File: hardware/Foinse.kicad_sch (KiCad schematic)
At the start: 81 parts, among them J1 ESQ-110-X-X-D, J15 39-29-1048, J3 PJ-063AH, J4 5023860570, J7 FAULT2, J8 FAULT1, Q1 IPD90P04P4L04ATMA1, Q2 IPD90P04P4L04ATMA1, U1 STM32F072C8Tx, U17 LTC4412xS6, U19 TPS56A37RPAR, U4 TJA1051T-3, U5 TPS563203, U6 ACS71240KEXBLT-010B3, U7 ACS71240KEXBLT-010B3

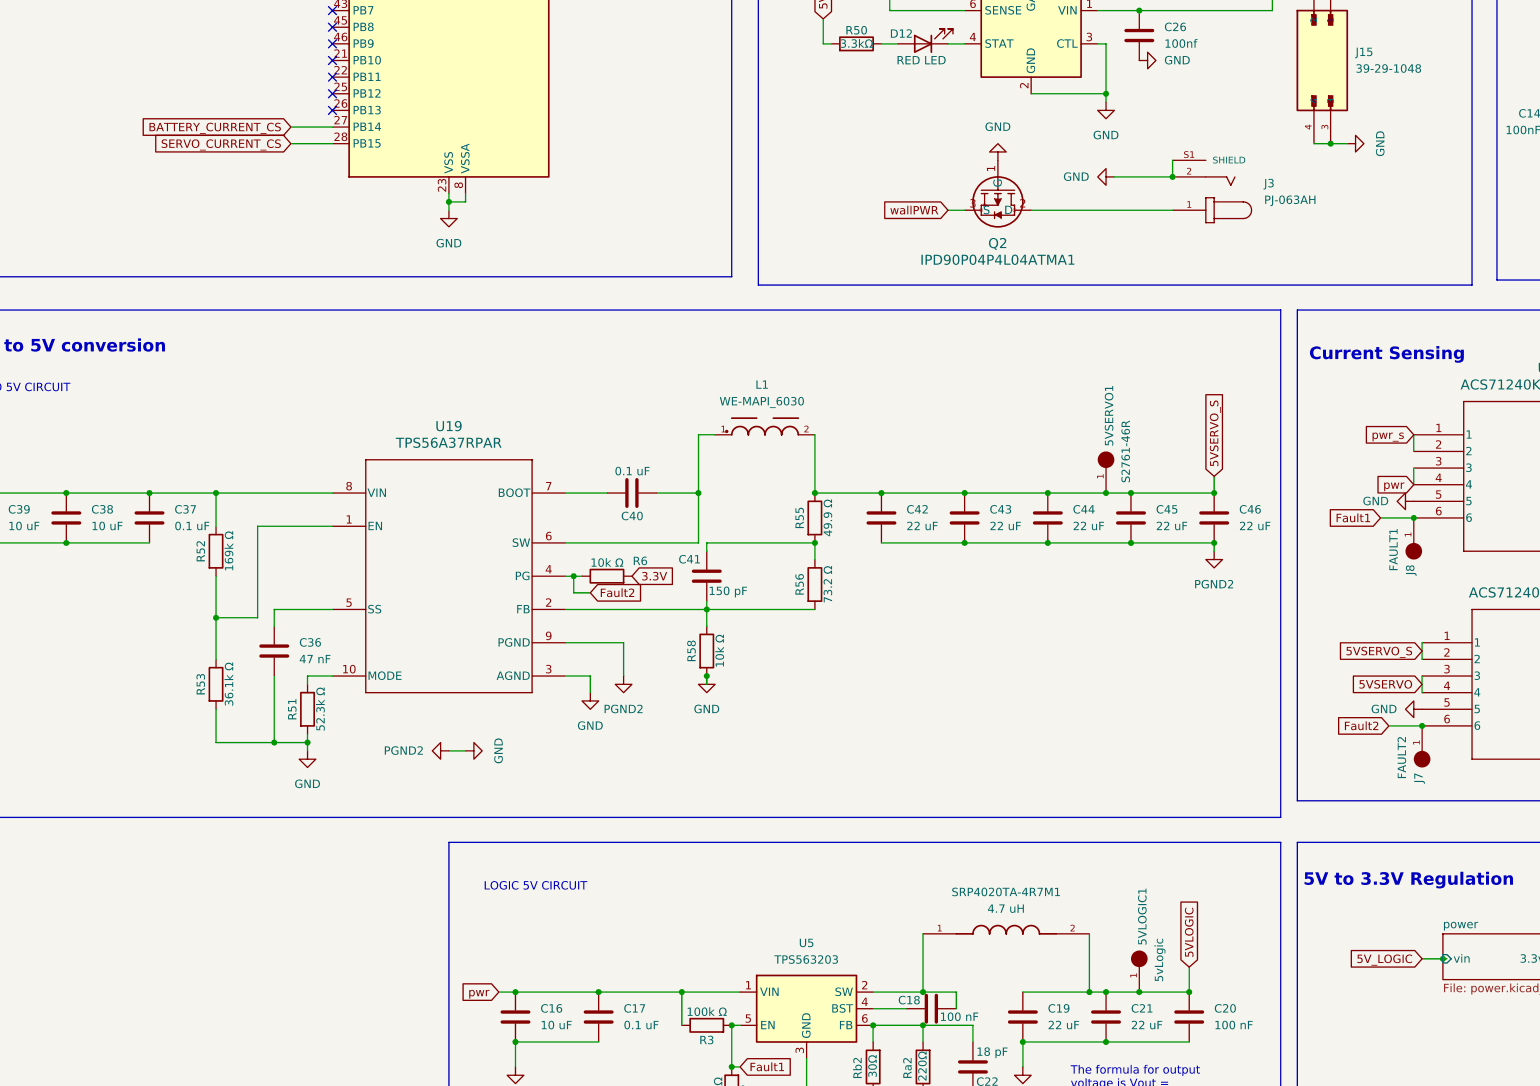
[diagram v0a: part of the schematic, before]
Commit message: minor changes
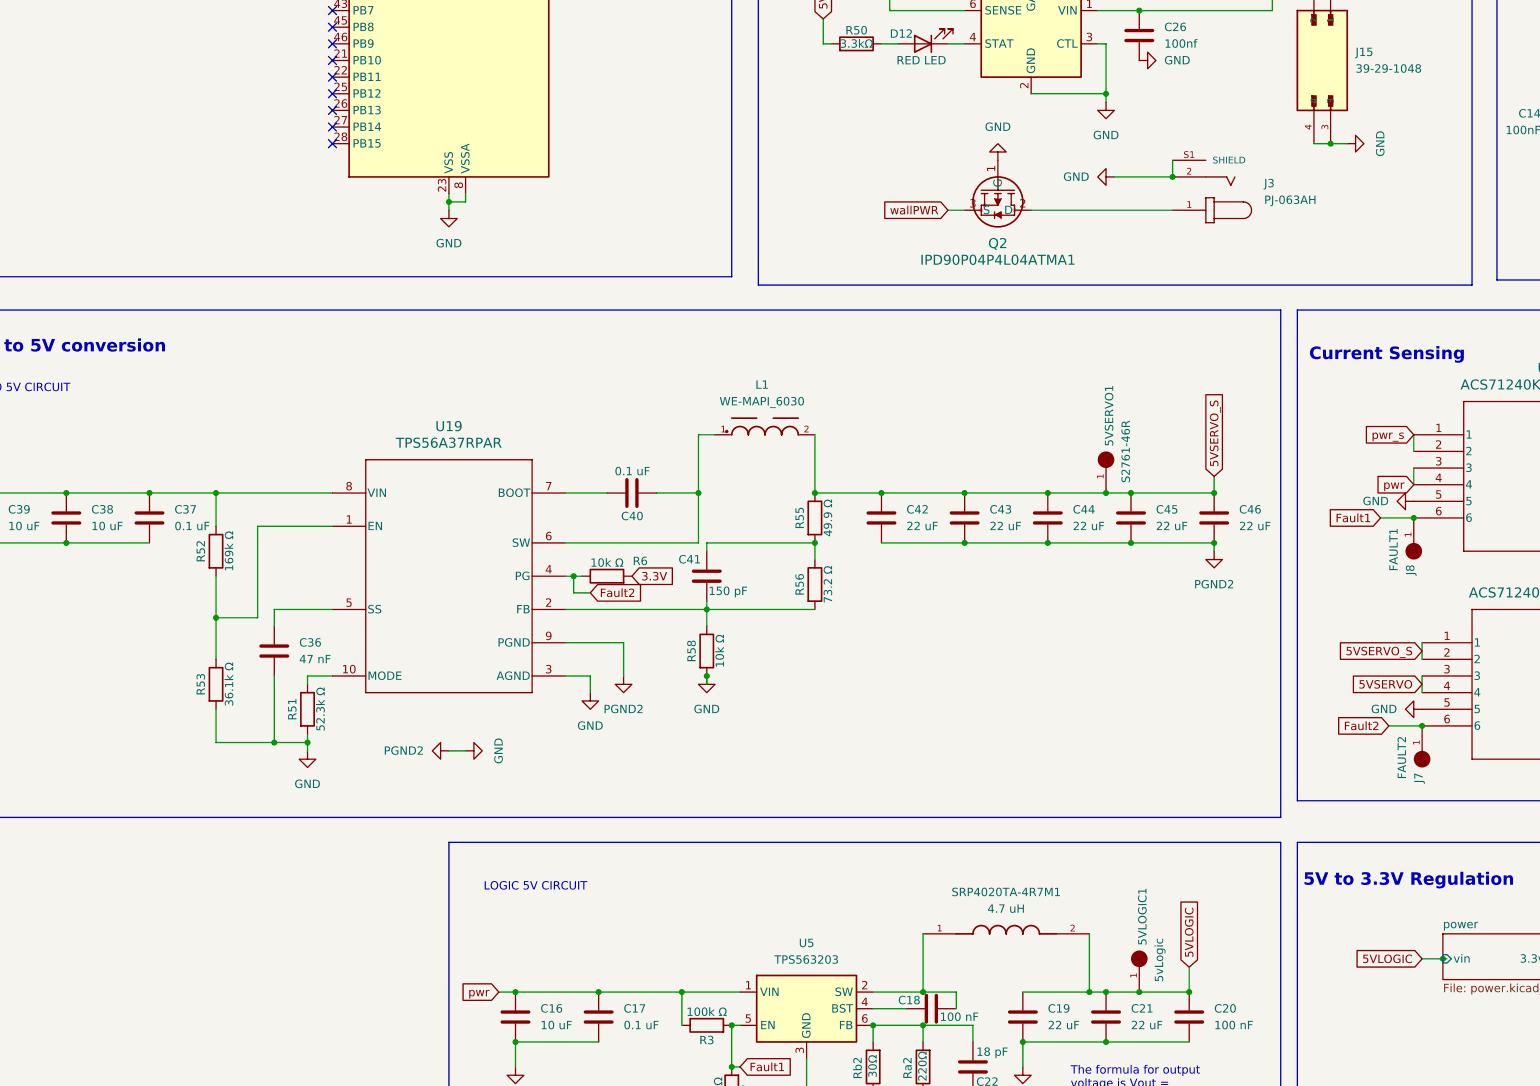
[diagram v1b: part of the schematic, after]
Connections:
- net BATTERY_CURRENT_CS: no longer names the net of U1.27 (PB14)
- net SERVO_CURRENT_CS: no longer names the net of U1.28 (PB15)
- no-connect marks 35 -> 37
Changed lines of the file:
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@@
 	)
 	(no_connect
+		(at 179.07 187.96)
+	)
+	(no_connect
 		(at 179.07 175.26)
 	)
@@
 	)
 	(no_connect
+		(at 179.07 185.42)
+	)
+	(no_connect
 		(at 386.08 269.24)
 	)
@@
 	(wire
 		(pts
-			(xy 172.72 185.42) (xy 179.07 185.42)
-		)
-		(stroke
-			(width 0)
-			(type default)
-		)
-	)
-	(wire
-		(pts
 			(xy 224.79 113.03) (xy 224.79 115.57)
 		)
@@
 	(wire
 		(pts
-			(xy 172.72 187.96) (xy 179.07 187.96)
-		)
-		(stroke
-			(width 0)
-			(type default)
-		)
-	)
-	(wire
-		(pts
 			(xy 151.13 102.87) (xy 165.1 102.87)
 		)
@@
 		)
 	)
-	(global_label "SERVO_CURRENT_CS"
-		(shape input)
-		(at 172.72 187.96 180)
-		(fields_autoplaced yes)
-		(effects
-			(font
-				(size 1.27 1.27)
-			)
-			(justify right)
-		)
-		(property "Intersheetrefs" "${INTERSHEET_REFS}"
-			(at 150.6849 187.96 0)
-			(effects
-				(font
-					(size 1.27 1.27)
-				)
-				(justify right)
-				(hide yes)
-			)
-		)
-	)
 	(global_label "CAN_-"
 		(shape input)
@@
 		)
 	)
-	(global_label "5V_LOGIC"
+	(global_label "5VLOGIC"
 		(shape input)
 		(at 345.44 312.42 180)
@@
 		)
 		(property "Intersheetrefs" "${INTERSHEET_REFS}"
-			(at 333.6857 312.42 0)
+			(at 334.6533 312.42 0)
 			(effects
 				(font
@@
 				(hide yes)
 			)
-		)
-	)
-	(global_label "BATTERY_CURRENT_CS"
-		(shape input)
-		(at 172.72 185.42 180)
-		(fields_autoplaced yes)
-		(effects
-			(font
-				(size 1.27 1.27)
-			)
-			(justify right)
-		)
-		(property "Intersheetrefs" "${INTERSHEET_REFS}"
-			(at 148.9311 185.42 0)
-			(effects
-				(font
-					(size 1.27 1.27)
-				)
-				(justify right)
-				(hide yes)
-			)
